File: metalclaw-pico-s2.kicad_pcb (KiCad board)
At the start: 2 copper layers, 3 parts, among them J1 USB_C_Receptacle_USB2.0_14P, U1 ESP32-S2

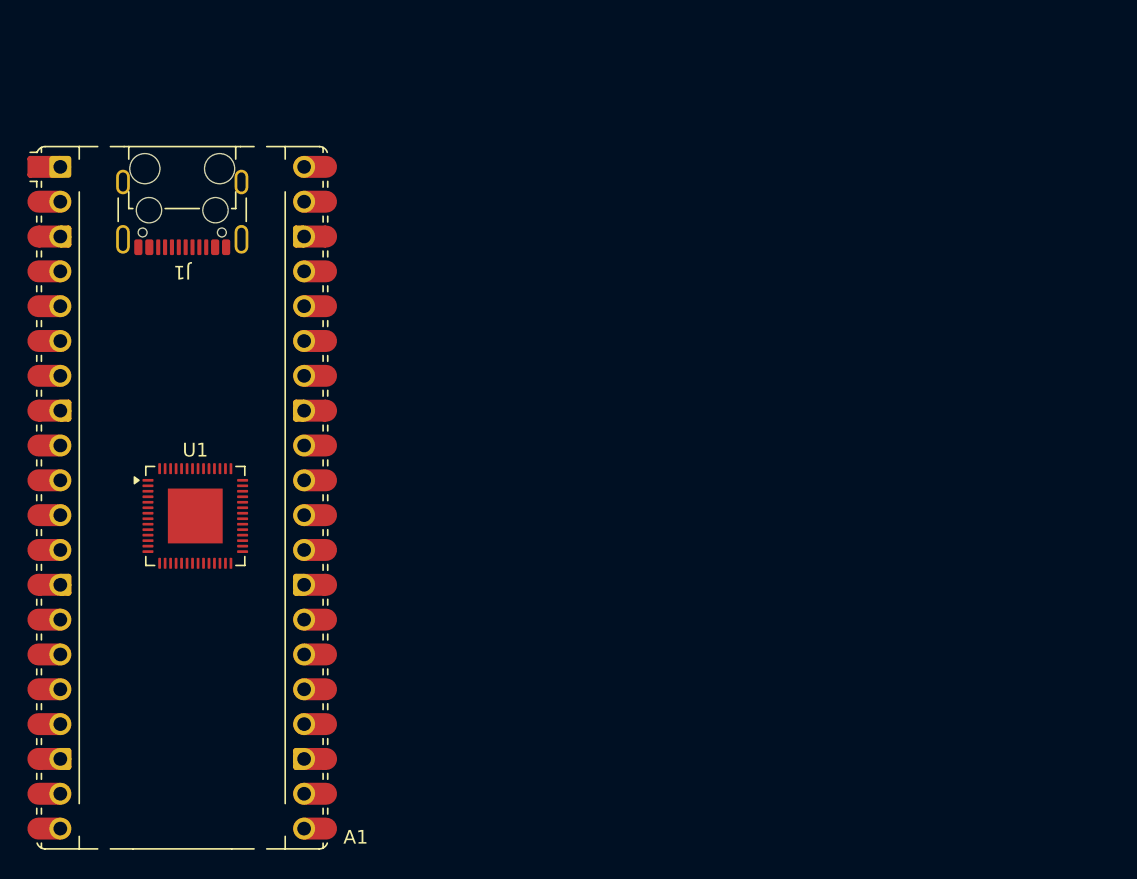
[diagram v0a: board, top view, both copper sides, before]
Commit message: Initial schematic connections
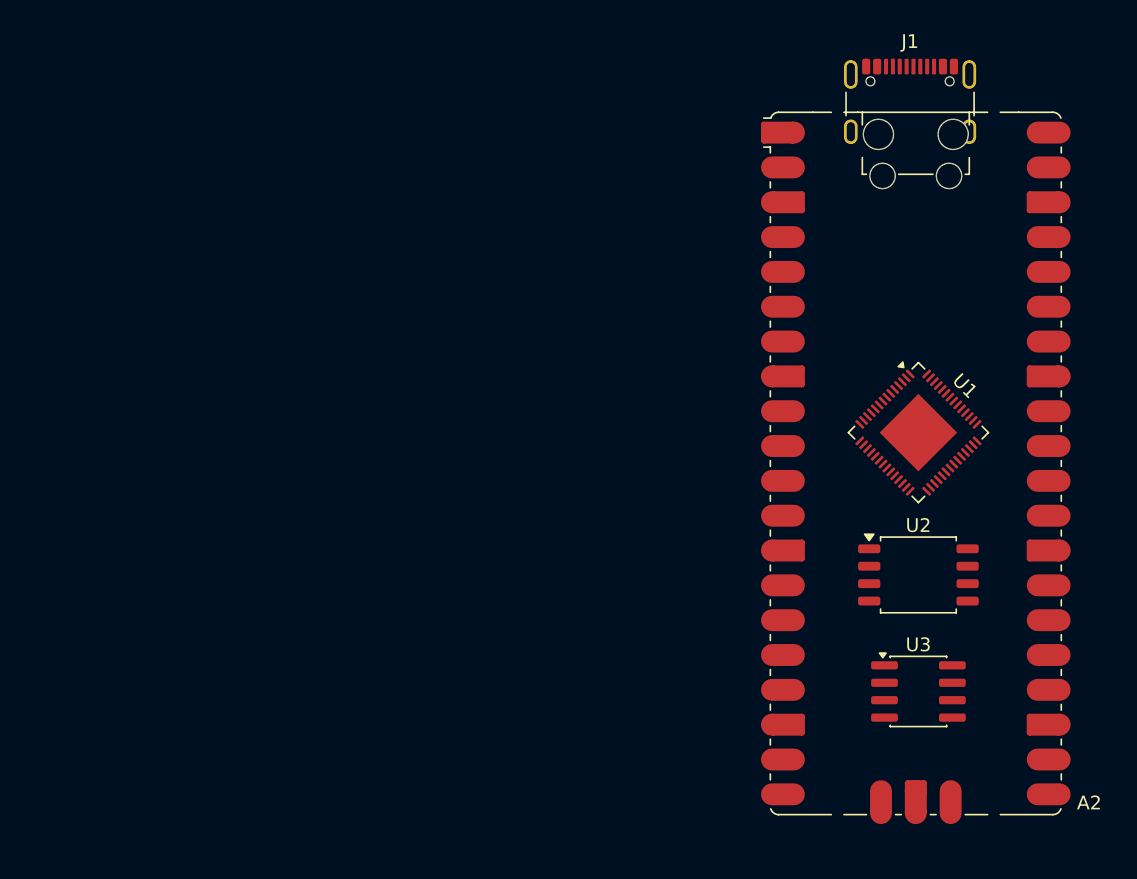
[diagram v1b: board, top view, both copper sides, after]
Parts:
- removed A1: RaspberryPi_Pico, Module:RaspberryPi_Pico_Common_Unspecified
- added A2: RaspberryPi_Pico, Module:RaspberryPi_Pico_SMD_HandSolder, F.Cu at (163.8, 98.9)
- added U2: W25Q16JVSS, Package_SO:SOIC-8_5.3x5.3mm_P1.27mm, F.Cu at (164.0, 107.0)
- added U3: APS6404L-3SQRx-SN, Package_SO:SOIC-8_3.9x4.9mm_P1.27mm, F.Cu at (164.0, 115.5)
- moved J1 53.4 mm to (163.4, 73.6), turned to 0 degrees
- moved U1 53.1 mm to (164.0, 96.6), turned to -45 degrees
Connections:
- J1 pad A1: Net-(J1-GND-PadA1) -> GND
- J1 pad A12: Net-(J1-GND-PadA1) -> GND
- J1 pad A6: unconnected-(J1-D+-PadA6) -> Net-(U1-GPIO20/USB_D+)
- J1 pad A7: unconnected-(J1-D--PadA7) -> Net-(U1-GPIO19/USB_D-)
- J1 pad B1: Net-(J1-GND-PadA1) -> GND
- J1 pad B12: Net-(J1-GND-PadA1) -> GND
- J1 pad B6: unconnected-(J1-D+-PadB6) -> /GP28
- J1 pad B7: unconnected-(J1-D--PadB7) -> Net-(U1-GPIO19/USB_D-)
- U1 pad 10: unconnected-(U1-GPIO5-Pad10) -> /GP5
- U1 pad 11: unconnected-(U1-GPIO6-Pad11) -> /GP6
- U1 pad 12: unconnected-(U1-GPIO7-Pad12) -> /GP7
- U1 pad 13: unconnected-(U1-GPIO8-Pad13) -> /GP8
- U1 pad 14: unconnected-(U1-GPIO9-Pad14) -> /GP9
- U1 pad 15: unconnected-(U1-GPIO10-Pad15) -> /GP10
- U1 pad 16: unconnected-(U1-GPIO11-Pad16) -> /GP11
- U1 pad 17: unconnected-(U1-GPIO12-Pad17) -> /GP12
- U1 pad 18: unconnected-(U1-GPIO13-Pad18) -> /GP13
- U1 pad 19: unconnected-(U1-GPIO14-Pad19) -> /GP14
- U1 pad 21: unconnected-(U1-XTAL_32K_P-Pad21) -> /RUN
- U1 pad 22: unconnected-(U1-XTAL_32K_N-Pad22) -> /3V3_EN
- U1 pad 23: unconnected-(U1-DAC_1-Pad23) -> /GP26
- U1 pad 24: unconnected-(U1-DAC_2-Pad24) -> /GP27
- U1 pad 25: unconnected-(U1-GPIO19/USB_D--Pad25) -> Net-(U1-GPIO19/USB_D-)
- U1 pad 26: unconnected-(U1-GPIO20/USB_D+-Pad26) -> Net-(U1-GPIO20/USB_D+)
- U1 pad 28: unconnected-(U1-GPIO21-Pad28) -> Net-(U1-GPIO21)
- U1 pad 29: unconnected-(U1-SPICS1-Pad29) -> Net-(U1-SPICS1)
- U1 pad 31: unconnected-(U1-SPIHD-Pad31) -> Net-(U1-SPIHD)
- U1 pad 32: unconnected-(U1-SPIWP-Pad32) -> Net-(U1-SPIWP)
- U1 pad 33: unconnected-(U1-SPICS0-Pad33) -> Net-(U1-SPICS0)
- U1 pad 34: unconnected-(U1-SPICLK-Pad34) -> Net-(U1-SPICLK)
- U1 pad 35: unconnected-(U1-SPIQ-Pad35) -> Net-(U1-SPIQ)
- U1 pad 36: unconnected-(U1-SPID-Pad36) -> Net-(U1-SPID)
- U1 pad 37: unconnected-(U1-GPIO33-Pad37) -> /GP15
- U1 pad 38: unconnected-(U1-GPIO34-Pad38) -> /GP16
- U1 pad 39: unconnected-(U1-GPIO35-Pad39) -> /GP17
- U1 pad 40: unconnected-(U1-GPIO36-Pad40) -> /GP18
- U1 pad 41: unconnected-(U1-GPIO37-Pad41) -> /GP20
- U1 pad 42: unconnected-(U1-GPIO38-Pad42) -> /GP19
- U1 pad 43: unconnected-(U1-MTCK-Pad43) -> /MTCK
- U1 pad 44: unconnected-(U1-MTD0-Pad44) -> /MTDO
- U1 pad 46: unconnected-(U1-MDTI-Pad46) -> /MTDI
- U1 pad 47: unconnected-(U1-MTMS-Pad47) -> /MTMS
- U1 pad 48: unconnected-(U1-U0TXD-Pad48) -> /SWCLK
- U1 pad 49: unconnected-(U1-U0RXD-Pad49) -> /SWDIO
- U1 pad 5: unconnected-(U1-GPIO0-Pad5) -> /GP0
- U1 pad 50: unconnected-(U1-GPIO45-Pad50) -> /GP21
- U1 pad 55: unconnected-(U1-GPIO46-Pad55) -> /GP22
- U1 pad 57: unconnected-(U1-GND-Pad57) -> GND
- U1 pad 6: unconnected-(U1-GPIO1-Pad6) -> /GP1
- U1 pad 7: unconnected-(U1-GPIO2-Pad7) -> /GP2
- U1 pad 8: unconnected-(U1-GPIO3-Pad8) -> /GP3
- U1 pad 9: unconnected-(U1-GPIO4-Pad9) -> /GP4
